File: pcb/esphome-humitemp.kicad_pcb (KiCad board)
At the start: 2 copper layers, 45 x 30 mm, 17 parts, among them J2 USB_IN, SW1 RESET, U1 SHT3x, U3 AMS1117-3.3, U4 ESP32-C3-MINI-1

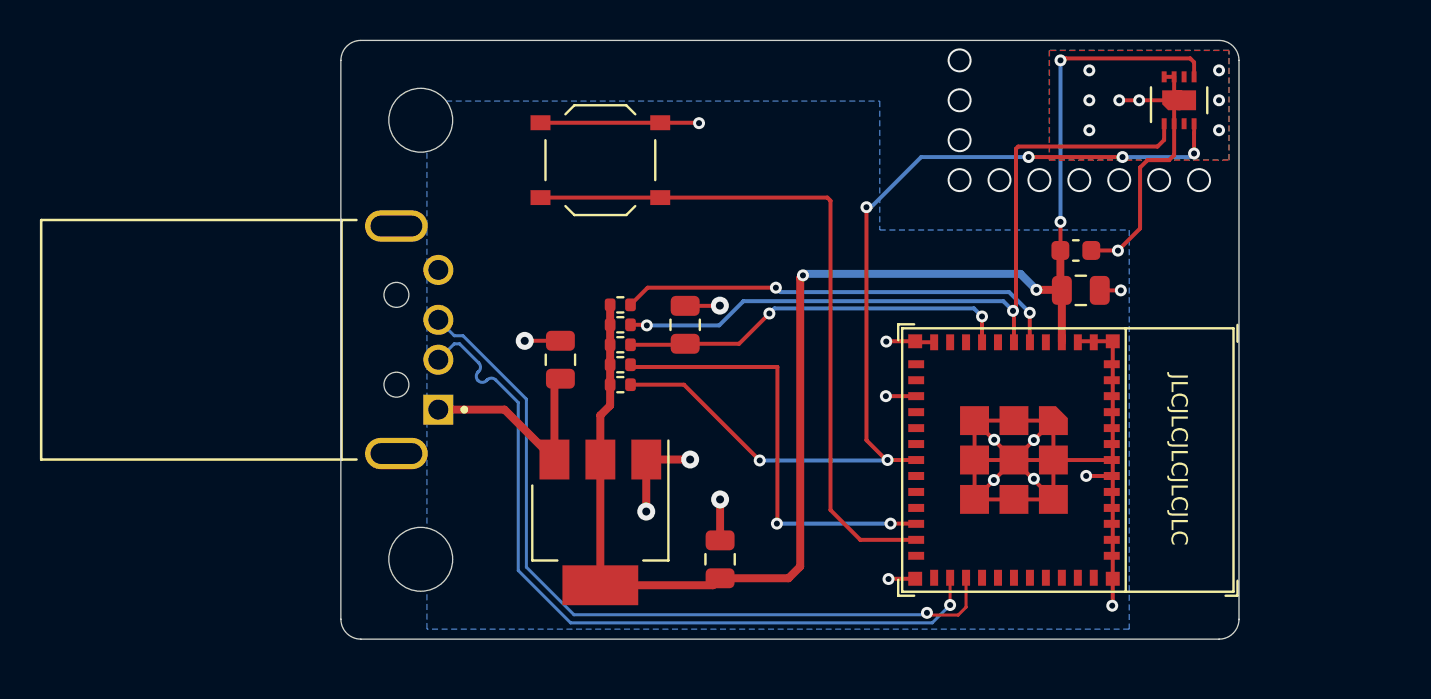
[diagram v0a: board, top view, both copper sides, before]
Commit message: v3
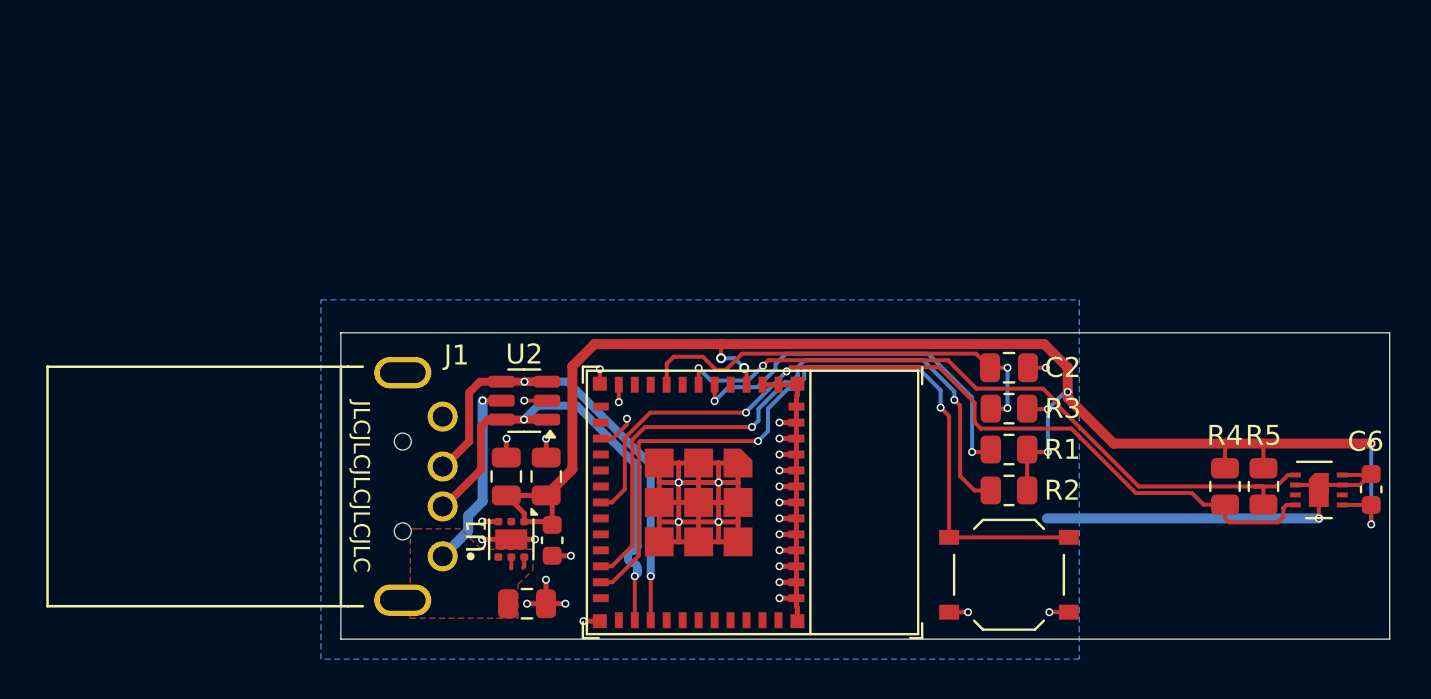
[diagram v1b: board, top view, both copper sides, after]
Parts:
- removed H1, H2: MountingHole, MountingHole:MountingHole_3.2mm_M3
- removed the U3 at (118.1, 74.6)
- added C6: 0.1u, Capacitor_SMD:C_0603_1608Metric, F.Cu at (156.8, 72.9)
- added U1: TLV75533PDRV, Package_SON:WSON-6-1EP_2x2mm_P0.65mm_EP1x1.6mm, F.Cu at (113.7, 75.4)
- added U2: USBLC6-4SC6, Package_TO_SOT_SMD:SOT-23-6, F.Cu at (114.3, 68.5)
- J1: renamed from J2; footprint esphome-humitemp:MOLEX_48037-0001 -> Project specific:SHOU_HAN_AM90
- R1: renamed from R5; footprint Resistor_SMD:R_0402_1005Metric -> Resistor_SMD:R_0805_2012Metric
- R2: renamed from R6; footprint Resistor_SMD:R_0402_1005Metric -> Resistor_SMD:R_0805_2012Metric
- R3: renamed from R4; footprint Resistor_SMD:R_0402_1005Metric -> Resistor_SMD:R_0805_2012Metric
- R4: renamed from R3; footprint Resistor_SMD:R_0402_1005Metric -> Resistor_SMD:R_0805_2012Metric
- R5: renamed from R2; footprint Resistor_SMD:R_0402_1005Metric -> Resistor_SMD:R_0805_2012Metric
- moved R5 33.2 mm to (151.4, 72.8), turned to -90 degrees
- moved R4 30.7 mm to (149.4, 72.8), turned to -90 degrees
- moved C1 30.3 mm to (113.4, 72.3), turned to -90 degrees
- moved C4 30.0 mm to (115.7, 75.5), turned to 90 degrees
- moved SW1 29.2 mm to (138.6, 77.2), turned to 0 degrees
- moved R1 20.8 mm to (138.6, 70.9), turned to 180 degrees
- moved U4 20.7 mm to (154.1, 73.0), turned to 0 degrees
- moved R2 20.5 mm to (138.6, 73.0), turned to 180 degrees
- moved R3 19.7 mm to (138.6, 68.9), turned to 180 degrees
- moved C2 16.4 mm to (138.6, 66.8), turned to 180 degrees
- moved U3 15.9 mm to (125.8, 73.6)
- moved C3 12.3 mm to (114.5, 78.7), turned to 0 degrees
- moved C5 9.65 mm to (115.4, 72.3)
- moved J1 7.36 mm to (108.2, 72.8)
- renumbered C6 to C1, C4 to C2, C1 to C3, C5 to C4, C2 to C5, U4 to U3, U1 to U4
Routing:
- net D-: track 39.2 -> 23.7 mm, vias 1 -> 2
- net D+: track 39.2 -> 24.2 mm, vias 1 -> 2
- net GND: track 90.4 -> 101.9 mm, vias 25 -> 34
- net Net-(U4-GPIO8): track 22.3 -> 32.5 mm
- net /GPIO0: track 35.0 -> 39.8 mm, vias 0 -> 2
- net SCL: track 48.1 -> 43.9 mm, vias 6 -> 2
- net Net-(U4-GPIO2/ADC1_CH2): track 22.4 -> 19.5 mm
- net +3V3: track 74.4 -> 76.8 mm, vias 4 -> 7
- net /EN: track 19.8 -> 22.3 mm
- net SDA: track 38.1 -> 35.7 mm
- net VBUS: track 11.0 -> 10.7 mm, vias 0 -> 1
- net (no net): vias 10 -> 0
- added copper zone on F.Cu, net VBUS
- removed copper zone on F.Cu, net GND
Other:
- board size 45 x 30 mm -> 52.5 x 15.3 mm
- board text added: "esphome-humitemp v2.1"
- board text removed: "<<hash>>"
- board text removed: "esphome-humitemp v2"

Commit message: Ready for final checking
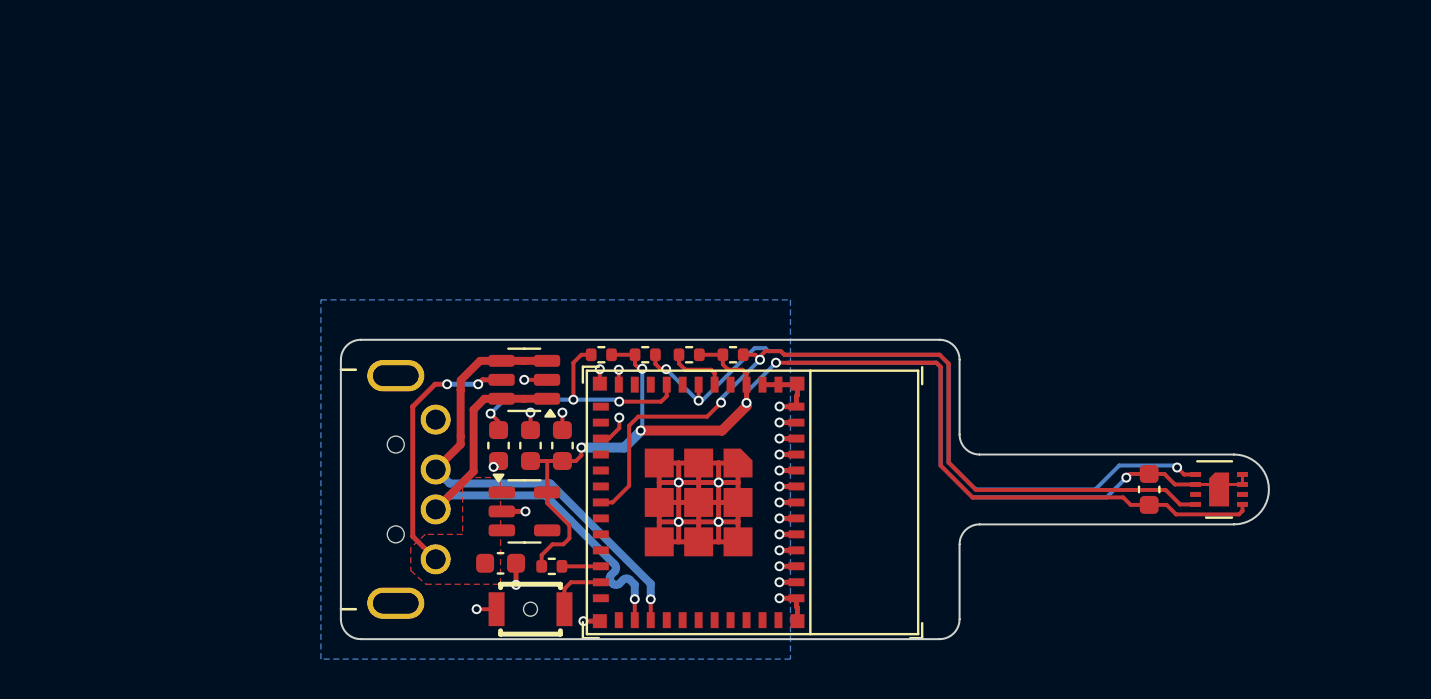
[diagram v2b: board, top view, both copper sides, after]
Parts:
- removed the C1 at (113.4, 72.3)
- removed the U1 at (113.7, 75.4)
- added REF**: Tab, PCM_kikit:Tab, F.Cu at (107.9, 80.4)
- added REF**: Tab, PCM_kikit:Tab, F.Cu at (107.9, 65.3)
- added REF**: Tab, PCM_kikit:Tab, F.Cu at (131.6, 80.4)
- added REF**: Tab, PCM_kikit:Tab, F.Cu at (131.6, 65.3)
- added U2: TLV75533PDBV, Package_TO_SOT_SMD:SOT-23-5, F.Cu at (114.3, 74.0)
- C1: renamed from C2; value 10u -> 1u; footprint Capacitor_SMD:C_0805_2012Metric -> Capacitor_SMD:C_0603_1608Metric
- C2: renamed from C3; value 1uF -> 10uF; footprint Capacitor_SMD:C_0805_2012Metric -> Capacitor_SMD:C_0603_1608Metric
- C4: renamed from C5; value 1uF -> 10uF; footprint Capacitor_SMD:C_0805_2012Metric -> Capacitor_SMD:C_0603_1608Metric
- R1, R2, R3, R4, R5: footprint Resistor_SMD:R_0805_2012Metric -> Resistor_SMD:R_0402_1005Metric
- SW1: footprint Button_Switch_SMD:SW_Push_1P1T_XKB_TS-1187A -> EasyEda:SW-SMD_L3.0-W2.5-P3.40-LS4.0-EH
- moved R5 31.7 mm to (120.4, 66.2), turned to 0 degrees
- moved C1 25.9 mm to (113.0, 70.7), turned to 90 degrees
- moved R4 25.5 mm to (124.8, 66.2), turned to 0 degrees
- moved SW1 24.0 mm to (114.6, 78.9), turned to 180 degrees
- moved R2 23.2 mm to (115.7, 76.8), turned to 0 degrees
- moved R3 20.6 mm to (118.2, 66.2)
- moved R1 16.7 mm to (122.6, 66.2)
- moved C5 11.1 mm to (145.6, 72.9)
- moved U4 5.00 mm to (149.1, 72.9)
- moved C3 4.87 mm to (114.6, 70.7), turned to -90 degrees
- moved C2 2.42 mm to (113.1, 76.6)
- moved C4 1.75 mm to (116.2, 70.7)
- moved U1 1.04 mm to (114.3, 67.4)
- moved J1 0.38 mm to (107.9, 72.9)
- renumbered C4 to C3, C6 to C5, U2 to U1
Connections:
- net /GPIO0 renamed Net-(SW1-A)
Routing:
- net Net-(SW1-A): track 39.8 -> 2.98 mm, vias 2 -> 0
- net Net-(U3-GPIO8): track 32.5 -> 1.95 mm, vias 2 -> 0
- net Net-(U3-GPIO2/ADC1_CH2): track 19.5 -> 3.00 mm, vias 2 -> 0
- net +3V3: track 76.8 -> 61.3 mm, vias 7 -> 5
- net /EN: track 22.3 -> 13.9 mm, vias 2 -> 3
- net GND: track 101.9 -> 94.9 mm, vias 34 -> 29
- net VBUS: track 10.7 -> 13.1 mm, vias 1 -> 2
- net SCL: track 43.9 -> 41.9 mm
- net SDA: track 35.7 -> 36.7 mm, vias 2 -> 3
- net D-: track 23.7 -> 24.6 mm, vias 2 -> 1
- net D+: track 24.2 -> 24.7 mm, vias 2 -> 1
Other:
- board size 52.5 x 15.3 mm -> 46.5 x 15 mm
- board text removed: "JLCJLCJLCJLCJLC"
- board text removed: "esphome-humitemp v2.1"
